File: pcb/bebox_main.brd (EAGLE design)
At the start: 92.8 x 35.2 mm, 29 parts, among them J1 SJ-435107RS, J2 SJ-435107RS, J4 SJ-435107RS, J6 PJ-102AH, P1 OSTTE020104, P2 OSTTE020104, P3 OSTTE020104, P4 OSTTE020104, P5 OSTTE020104, T1 TIP122, T2 TIP122, T3 TIP122, T4 TIP122, T5 TIP122

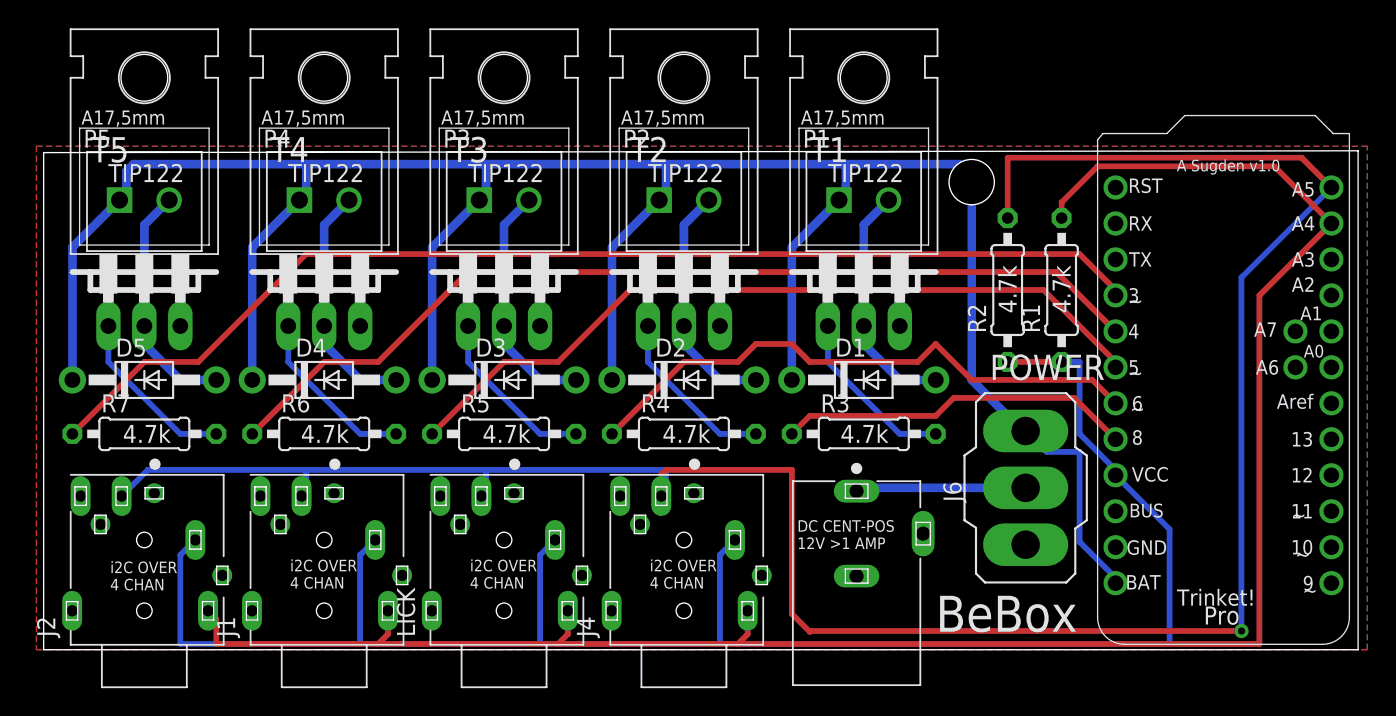
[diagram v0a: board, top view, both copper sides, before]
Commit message: Updated the boards.
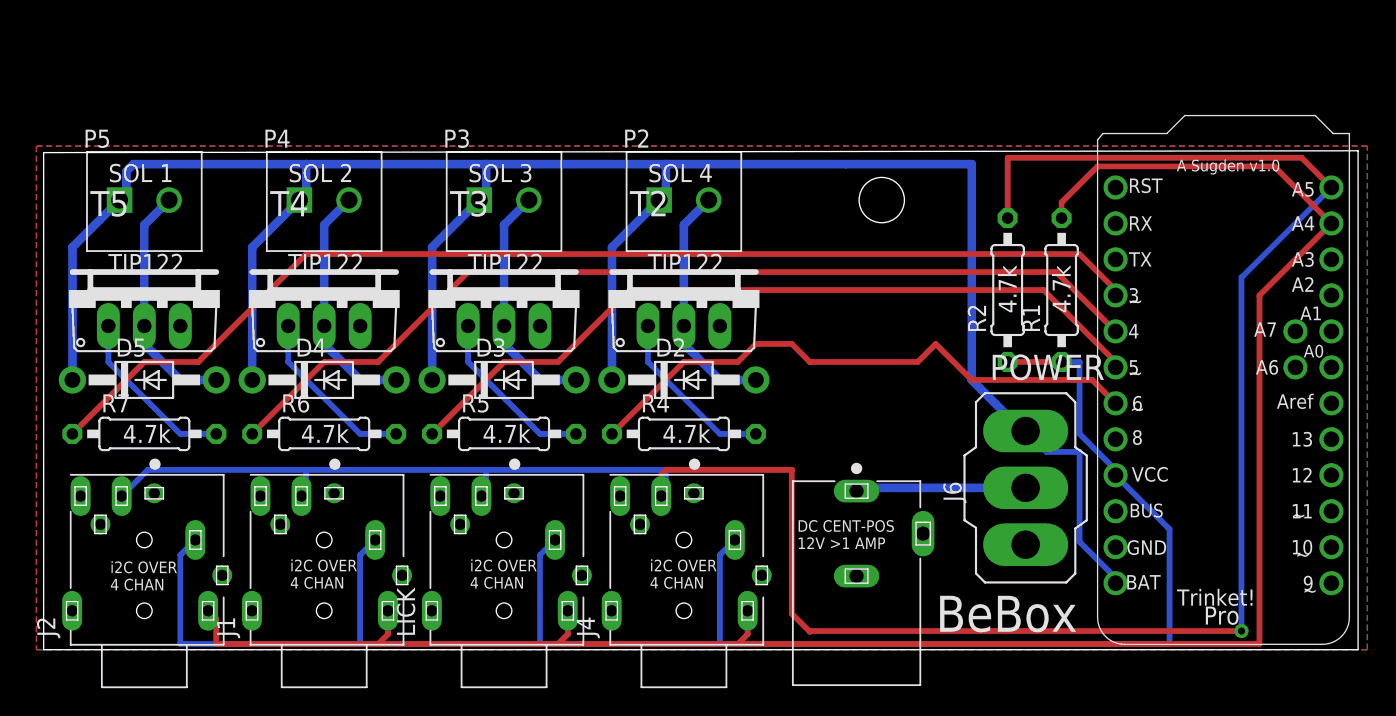
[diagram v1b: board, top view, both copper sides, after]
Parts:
- removed D1: 1N4004, adafruit:DO41-10
- removed P1: OSTTE020104, OSTTE020104:OST_OSTTE020104
- removed R3: 4.7k, rcl:0207/10
- removed T1: TIP122, transistor-neu-to92:TO220
- T2, T3, T4, T5: value TIP122 -> 2SC2098V; device transistor-neu-to92:TO220 -> transistor:TO220AV
- moved T2 3.81 mm to (54.6, 35.6)
- moved T3 3.81 mm to (41.9, 35.6)
- moved T4 3.81 mm to (29.2, 35.6)
- moved T5 3.81 mm to (16.5, 35.6)
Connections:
- removed net N$16: R3.1, U$1.8
- removed net N$2: R3.2, T1.1
- removed net N$3: D1.A, P1.2, T1.2
- net 12V: no longer D1.C, P1.1
- net GND: no longer T1.3
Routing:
- net N$16: track 25.1 -> 0.00 mm
- net N$3: track 17.0 -> 0.00 mm
- net 12V: track 178.8 -> 162.0 mm
- net N$2: track 12.3 -> 0.00 mm
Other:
- board text added: "SOL 1"
- board text added: "SOL 2"
- board text added: "SOL 3"
- board text added: "SOL 4"
